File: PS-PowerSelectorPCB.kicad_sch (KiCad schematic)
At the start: 11 parts, among them J1 SuppChargerIn, J2 PowerSupplyIn, J3 Conn_01x02, J4 Ext_Power, J5 Conn_01x02, SW1 Power Source Selector

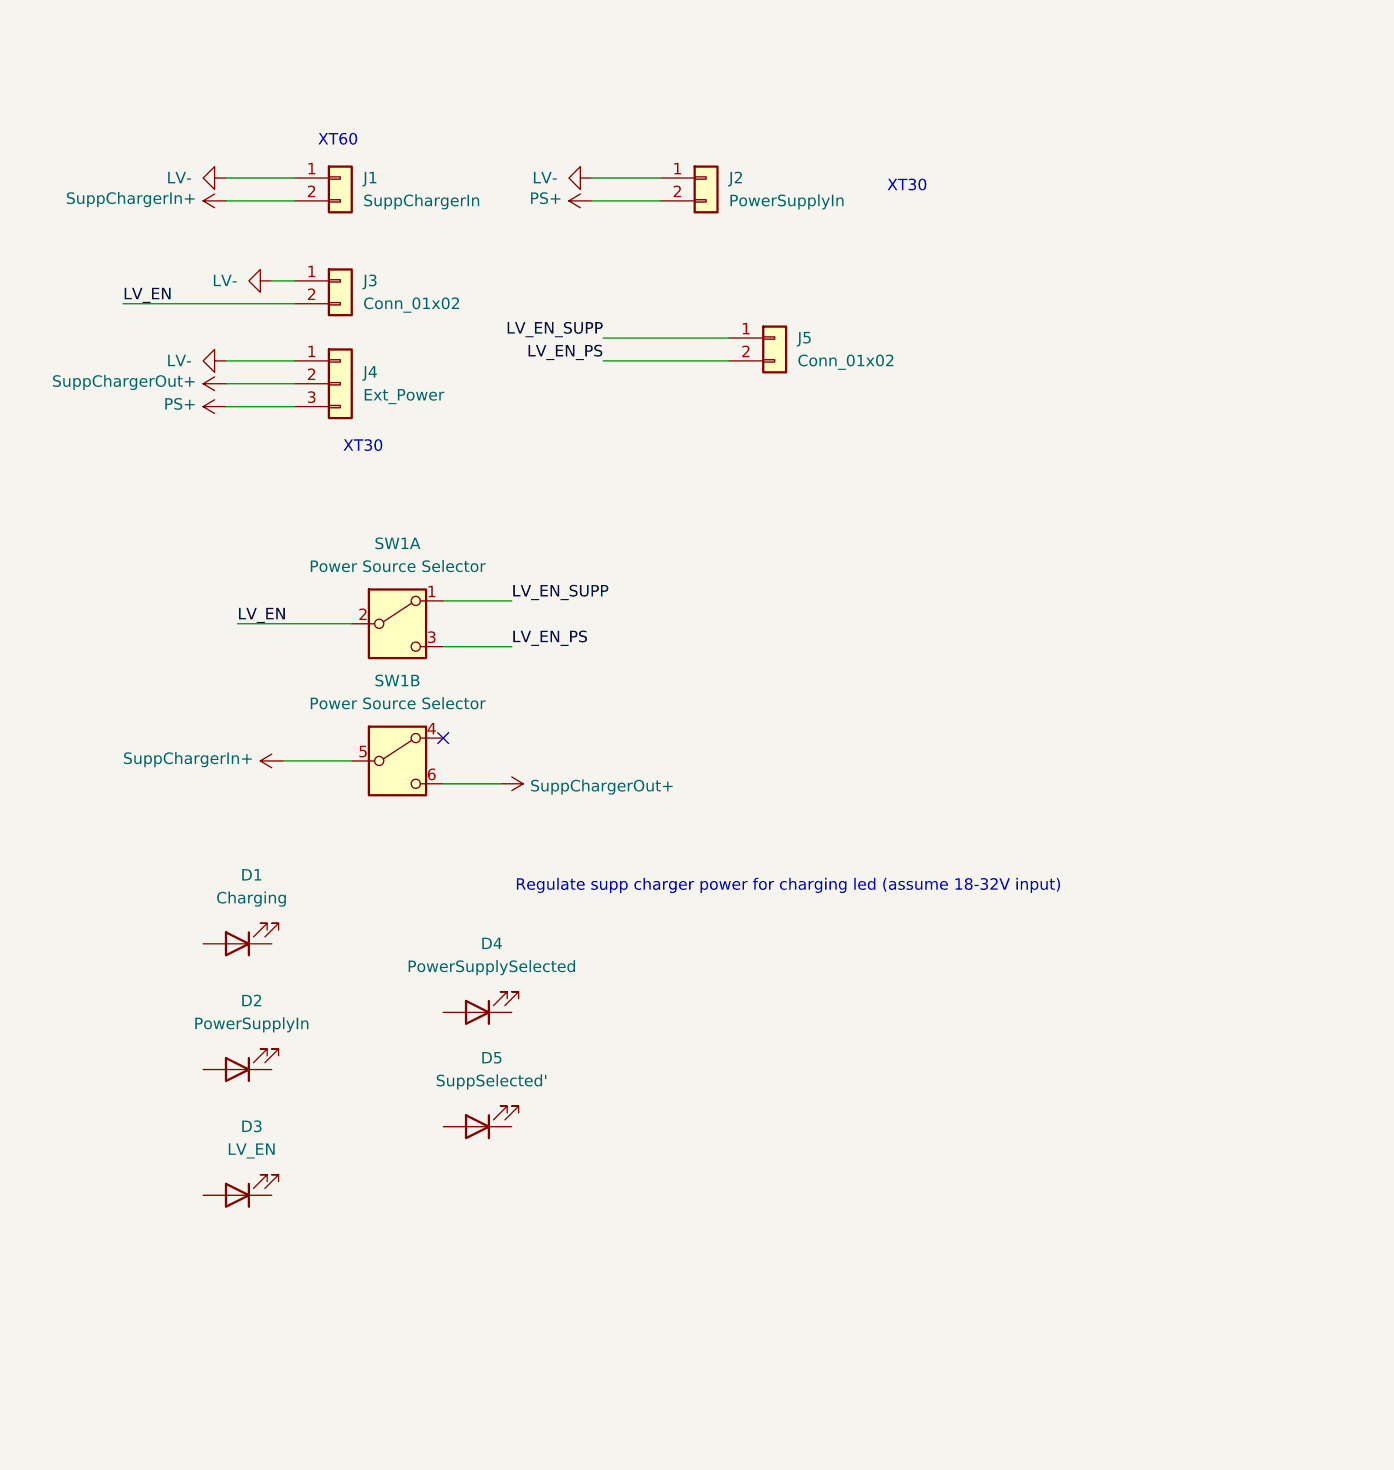
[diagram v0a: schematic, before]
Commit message: initial schematic
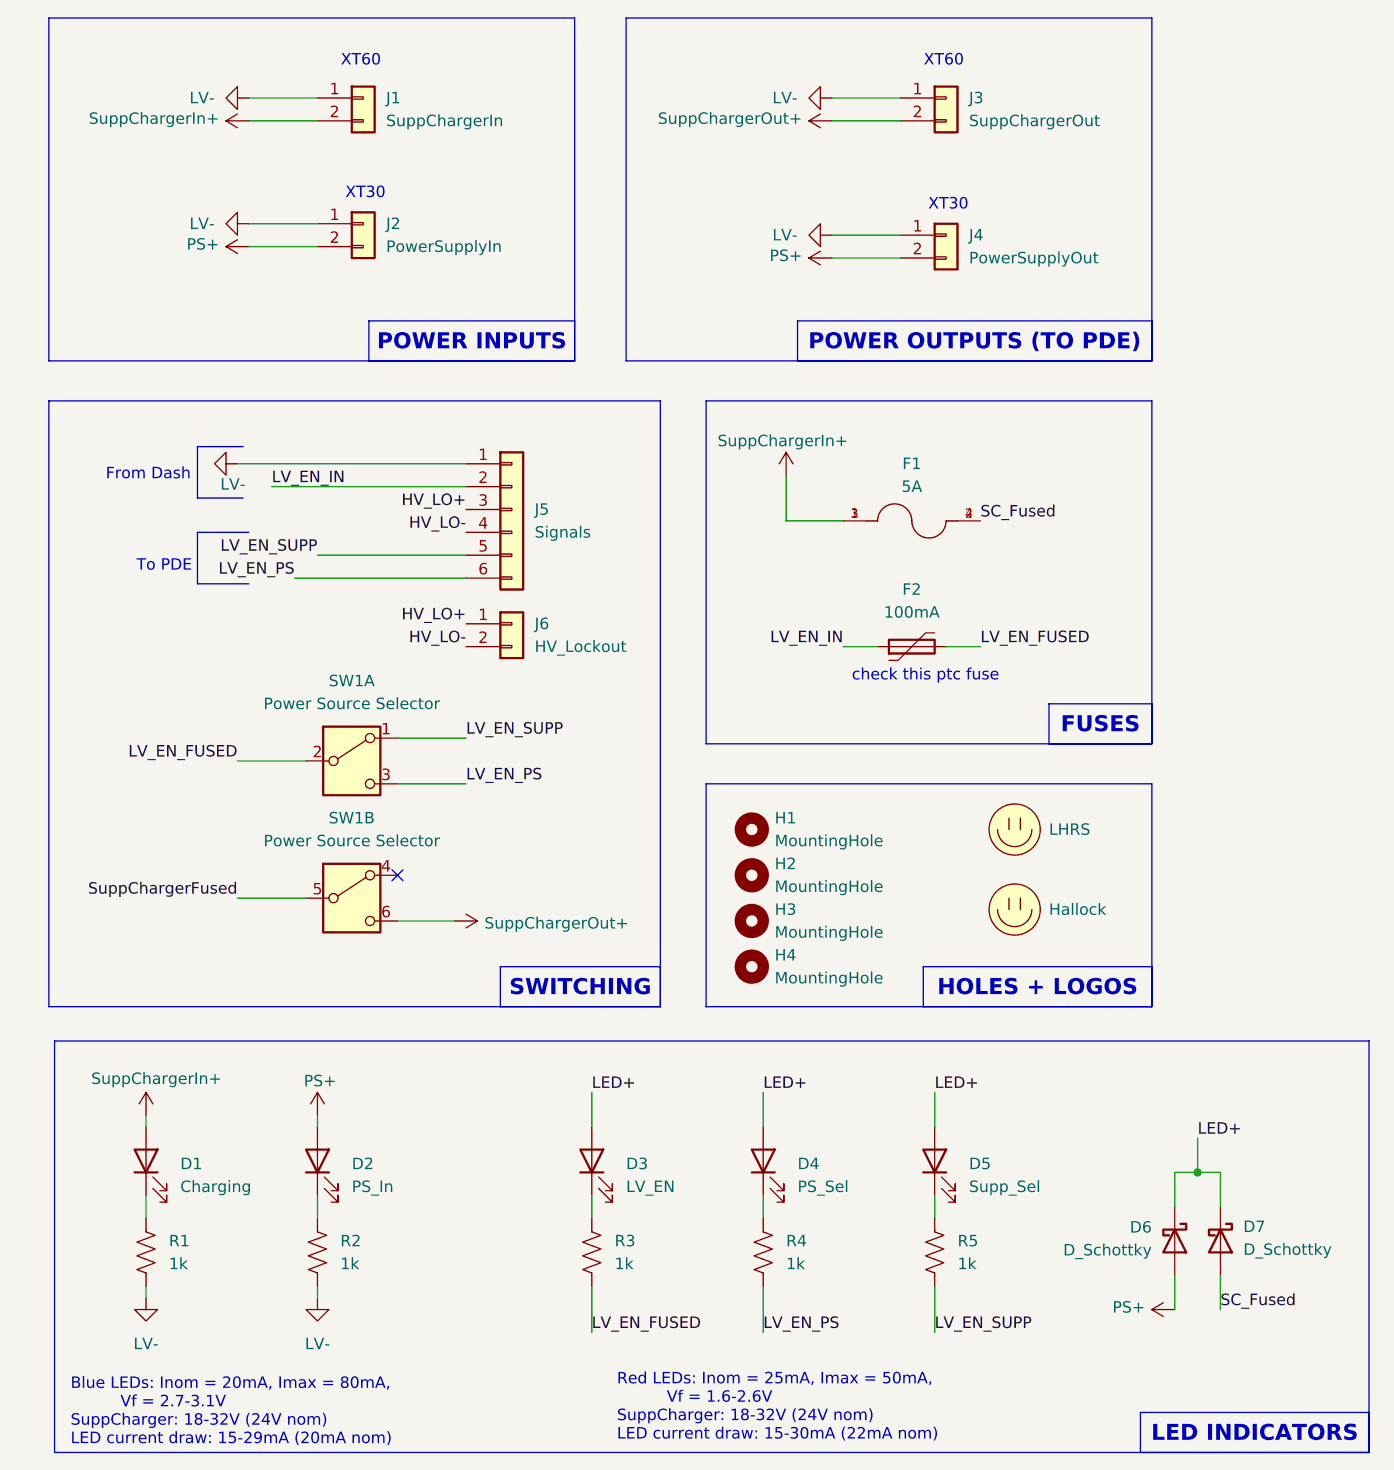
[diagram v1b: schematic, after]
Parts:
- removed J4: Ext_Power, symbol Connector_Generic:Conn_01x03
- removed J5: Conn_01x02, symbol Connector_Generic:Conn_01x02
- added D6, D7: D_Schottky, symbol Device:D_Schottky
- added F1: 5A, footprints:FUSE_3568, symbol 3568:3568
- added F2: 100mA, symbol Device:Polyfuse
- added H1, H2, H3, H4: MountingHole, MountingHole:MountingHole_3.2mm_M3, symbol Mechanical:MountingHole
- added J4: PowerSupplyOut, UTSVT_Connectors:AMASS_XT30PW-M_1x02_P2.50mm_Horizontal, symbol Connector_Generic:Conn_01x02
- added J5: Signals, Connector_Molex:Molex_Nano-Fit_105309-xx06_1x06_P2.50mm_Vertical, symbol Connector_Generic:Conn_01x06
- added J6: HV_Lockout, UTSVT_Connectors:Molex_Nano-Fit_105309-xx02_1x02_P2.50mm_Vertical, symbol Connector_Generic:Conn_01x02
- added LOGO1: LHRS, UTSVT_Logos:LHRs_LOGO, symbol utsvt_misc:Logo_Placeholder
- added LOGO2: Hallock, UTSVT_Logos:Hallock_Image_Tiny, symbol utsvt_misc:Logo_Placeholder
- added R1, R2, R3, R4, R5: 1k, symbol Device:R_US
- D2: value PowerSupplyIn -> PS_In
- D4: value PowerSupplySelected -> PS_Sel
- D5: value SuppSelected' -> Supp_Sel
- J1: footprint (none) -> Connector_AMASS:AMASS_XT60-M_1x02_P7.20mm_Vertical
- J2: footprint (none) -> UTSVT_Connectors:AMASS_XT30PW-M_1x02_P2.50mm_Horizontal
- J3: value Conn_01x02 -> SuppChargerOut; footprint (none) -> Connector_AMASS:AMASS_XT60-M_1x02_P7.20mm_Vertical
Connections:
- net LV-: now also J4.1 (Pin_1), J5.1 (Pin_1), R1.2, R2.2
- net LV_EN_PS: now also J5.6 (Pin_6), R4.2
- net LV_EN_SUPP: now also J5.5 (Pin_5), R5.2
- net PS+: now also D2.2 (A), D6.2 (A), J4.2 (Pin_2)
- net SuppChargerIn+: now also D1.2 (A), F1.1, F1.3; no longer SW1.5 (B)
- net SuppChargerOut+: now also J3.2 (Pin_2)
- net at D5.1 (K): now also R5.1
- net LED+: now reaches D5.2 (A)
- net LED+: now also D3.2 (A), D4.2 (A), D6.1 (K), D7.1 (K)
- net at D2.1 (K): now also R2.1
- net at D4.1 (K): now also R4.1
- net at D3.1 (K): now also R3.1
- net at D1.1 (K): now also R1.1
- net LV_EN renamed LV_EN_FUSED
- net LV_EN_FUSED: now also F2.2, R3.2; no longer J3.2 (Pin_2)
- new net HV_LO+: J5.3 (Pin_3), J6.1 (Pin_1)
- new net HV_LO-: J5.4 (Pin_4), J6.2 (Pin_2)
- new net LV_EN_IN: F2.1, J5.2 (Pin_2)
- new net SC_Fused: D7.2 (A), F1.2, F1.4
- new net SuppChargerFused: SW1.5 (B)
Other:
- note added: "Blue LEDs: Inom = 20mA, Imax = 80mA, Vf = 2.7-3.1V SuppCharger: 18-32V (24V nom) LED current draw: 15-29mA (20mA nom)"
- note added: "From Dash"
- note added: "Red LEDs: Inom = 25mA, Imax = 50mA, Vf = 1.6-2.6V SuppCharger: 18-32V (24V nom) LED current draw: 15-30mA (22mA nom)"
- note added: "To PDE"
- note added: "check this ptc fuse"
- note removed: "Regulate supp charger power for charging led (assume 18-32V input)"
- moved on the sheet: D1, D2, D3, D4, D5, SW1A, SW1B
